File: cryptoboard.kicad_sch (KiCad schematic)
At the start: 3 parts, among them J1 USB_A, U1 STM32F103C8Tx

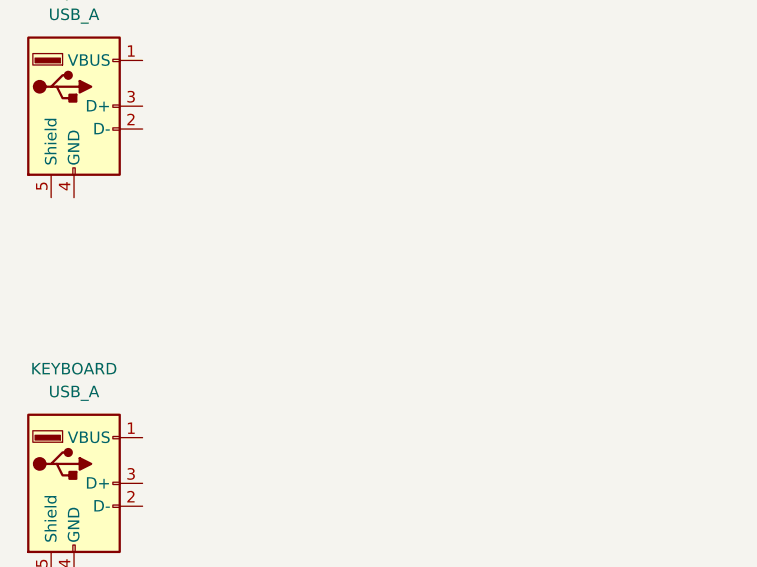
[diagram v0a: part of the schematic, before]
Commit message: add resistor
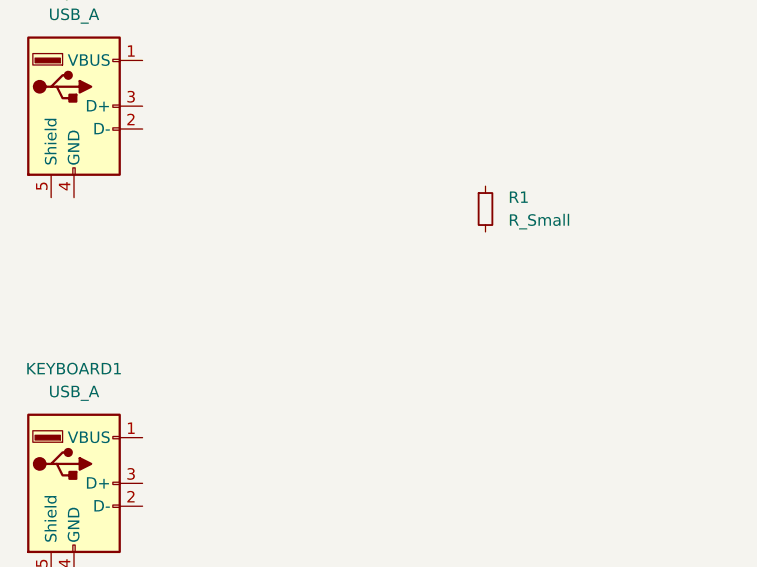
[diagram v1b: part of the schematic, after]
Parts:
- added R1: R_Small, symbol Device:R_Small
- J1: footprint (none) -> Connector_USB:USB_Micro-B_Molex-105017-0001
- KEYBOARD1: renamed from KEYBOARD; footprint (none) -> Connector_USB:USB_A_TE_292303-7_Horizontal
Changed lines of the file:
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@@
   (symbol (lib_id "Connector:USB_A") (at 22.86 69.85 0) (unit 1)
     (in_bom yes) (on_board yes) (dnp no) (fields_autoplaced)
-    (property "Reference" "KEYBOARD" (at 22.86 57.15 0)
+    (property "Reference" "KEYBOARD1" (at 22.86 57.15 0)
       (effects (font (size 1.27 1.27)))
     )
@@
       (effects (font (size 1.27 1.27)))
     )
-    (property "Footprint" "" (at 26.67 71.12 0)
+    (property "Footprint" "Connector_USB:USB_A_TE_292303-7_Horizontal" (at 26.67 71.12 0)
       (effects (font (size 1.27 1.27)) hide)
     )
@@
       (project "cryptoboard"
         (path "/dcd2214c-a8e3-4da9-953a-c4b4305fce7d"
-          (reference "KEYBOARD") (unit 1)
+          (reference "KEYBOARD1") (unit 1)
         )
       )
@@
       (effects (font (size 1.27 1.27)))
     )
-    (property "Footprint" "" (at 26.67 29.21 0)
+    (property "Footprint" "Connector_USB:USB_Micro-B_Molex-105017-0001" (at 26.67 29.21 0)
       (effects (font (size 1.27 1.27)) hide)
     )
@@
         )
       )
+    )
+  )
+  (symbol (lib_id "Device:R_Small") (at 68.58 39.37 0) (unit 1)
+    (in_bom yes) (on_board yes) (dnp no) (fields_autoplaced)
+    (property "Reference" "R1" (at 71.12 38.1 0)
+      (effects (font (size 1.27 1.27)) (justify left))
+    )
+    (property "Value" "R_Small" (at 71.12 40.64 0)
+      (effects (font (size 1.27 1.27)) (justify left))
+    )
+    (property "Footprint" "" (at 68.58 39.37 0)
+      (effects (font (size 1.27 1.27)) hide)
+    )
+    (property "Datasheet" "~" (at 68.58 39.37 0)
+      (effects (font (size 1.27 1.27)) hide)
+    )
+    (pin "1")
+    (pin "2")
+    (instances
+      (project "cryptoboard"
+        (path "/dcd2214c-a8e3-4da9-953a-c4b4305fce7d"
+          (reference "R1") (unit 1)
+        )
+      )
